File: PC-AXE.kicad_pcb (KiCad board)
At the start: 6 copper layers, 312 x 111.2 mm, 565 parts, among them J1 PCIexpress_bracket, J10 61900411021, J2 PCIexpress_x4, J3 353180620, J4 353180620, J5 353180620, J6 Conn_01x06, J7 61900411021, J8 61900411021, J9 61900411021, U1 TLV62568ADRLR, U10 CSD95472Q5MC, U11 CSD95472Q5MC, U12 CSD95472Q5MC, U13 25MHz, U14 TXU0304PW, U15 MCP1824T-0802E, U16 MCP1824T-1202E, U17 BM1370_mode1, U18 BM1370_mode1, U19 BM1370_mode1, U2 AP2204K-1.8, U20 BM1370_mode1, U21 BM1370_mode1, U22 BM1370_mode1, U23 BM1370_mode1, U24 BM1370_mode1, U25 BM1370_mode1, U26 BM1370_mode1, U27 BM1370_mode1, U28 BM1370_mode1, U29 EMC2305, U3 VL805, U30 M93C46-WDW6TP, U31 FT4232HQ, U4 W25Q32JVZP, U5 AP3211, U6 TPS53667RTAR, U7 CSD95472Q5MC, U8 CSD95472Q5MC, U9 CSD95472Q5MC, Y1 25Mhz, Y2 12MHz

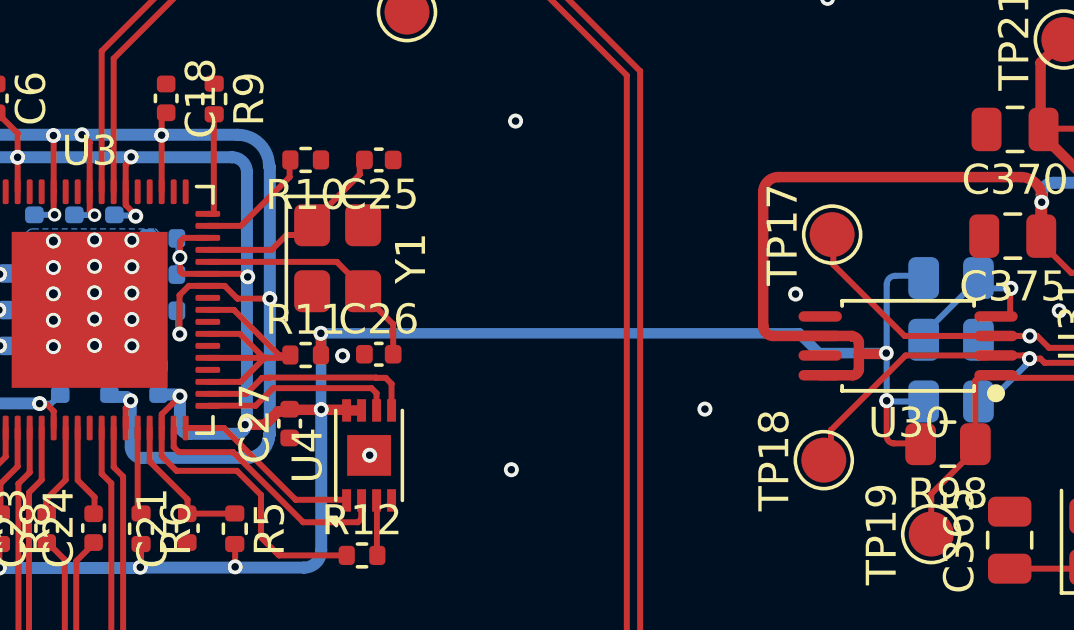
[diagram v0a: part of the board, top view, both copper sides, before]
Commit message: update
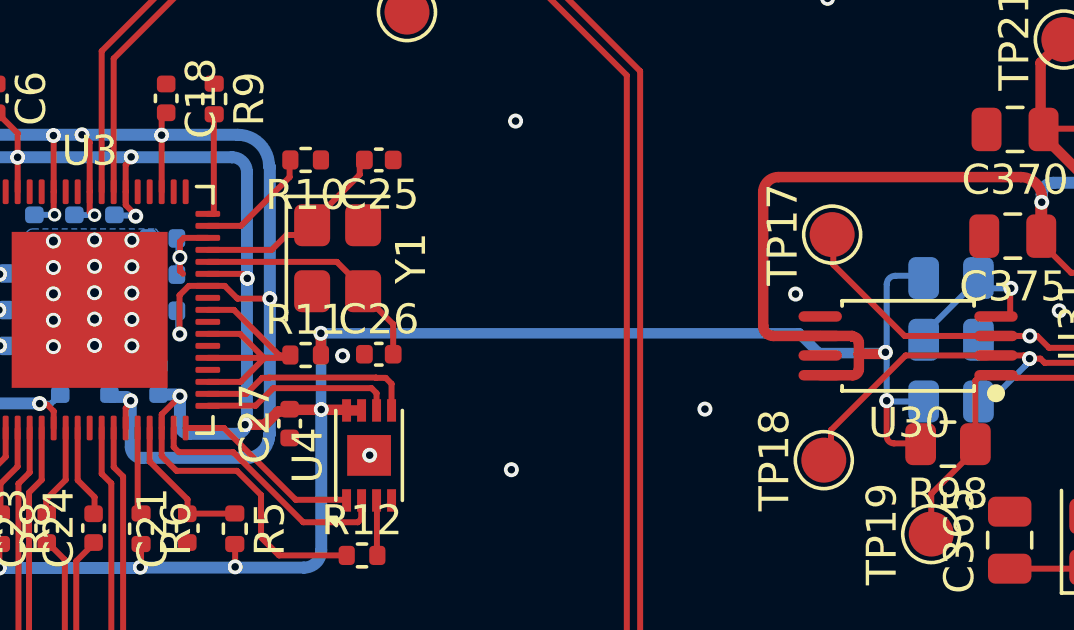
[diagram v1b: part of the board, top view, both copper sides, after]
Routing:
- net +3V3: track 719.4 -> 718.7 mm
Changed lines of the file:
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@@
+	)
+	(segment
+		(start 169.431272 167.71143)
+		(end 169.380002 167.7627)
+		(width 0.35)
+		(layer "F.Cu")
+		(net 16)
+	)
+	(segment
+		(start 169.380002 167.7627)
+		(end 168.54492 167.7627)
+		(width 0.35)
+		(layer "F.Cu")
+		(net 16)
 	)
 	(segment
@@
 	)
 	(segment
-		(start 168.54492 167.7627)
-		(end 169.43392 167.7627)
-		(width 0.35)
-		(layer "F.Cu")
-		(net 16)
-	)
-	(segment
 		(start 136.46472 168.7152)
 		(end 136.48352 168.6964)
@@
 	)
 	(segment
+		(start 146.84342 165.0964)
+		(end 148.01142 165.0964)
+		(width 0.2)
+		(layer "F.Cu")
+		(net 16)
+	)
+	(segment
 		(start 169.71332 170.7472)
 		(end 170.71662 170.7472)
@@
 	)
 	(segment
-		(start 146.01674 165.0957)
-		(end 148.07252 165.0957)
-		(width 0.2)
-		(layer "F.Cu")
-		(net 16)
-	)
-	(segment
 		(start 147.81239 171.6616)
 		(end 148.61862 172.46783)
@@
 	)
 	(segment
+		(start 169.431272 167.71143)
+		(end 169.45968 167.739838)
+		(width 0.35)
+		(layer "F.Cu")
+		(net 16)
+	)
+	(segment
 		(start 115.65852 123.747)
 		(end 117.21785 125.30633)
@@
 	)
 	(segment
+		(start 148.01142 165.0964)
+		(end 148.16142 165.2464)
+		(width 0.2)
+		(layer "F.Cu")
+		(net 16)
+	)
+	(segment
 		(start 165.35722 166.8229)
 		(end 165.35722 162.3779)
@@
 	)
 	(via
-		(at 169.45932 167.7373)
+		(at 169.431272 167.71143)
 		(size 0.5)
 		(drill 0.25)
@@
 	)
 	(via
-		(at 148.17412 165.1973)
+		(at 148.16142 165.2464)
 		(size 0.5)
 		(drill 0.25)
@@
 	)
 	(arc
+		(start 169.45968 167.739838)
+		(mid 169.450965 167.756113)
+		(end 169.43392 167.7627)
+		(width 0.35)
+		(layer "F.Cu")
+		(net 16)
+	)
+	(arc
 		(start 267.73192 180.8945)
 		(mid 267.085342 180.626678)
@@
 	)
 	(arc
-		(start 169.45932 167.7373)
-		(mid 169.451881 167.755261)
-		(end 169.43392 167.7627)
-		(width 0.35)
-		(layer "F.Cu")
-		(net 16)
-	)
-	(arc
 		(start 147.75502 174.1381)
 		(mid 147.765593 174.112573)
@@
 		(width 0.2)
 		(layer "F.Cu")
-		(net 16)
-	)
-	(arc
-		(start 148.07252 165.0957)
-		(mid 148.135382 165.121738)
-		(end 148.16142 165.1846)
-		(width 0.2)
-		(layer "F.Cu")
